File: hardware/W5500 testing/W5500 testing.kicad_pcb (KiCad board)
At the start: 2 copper layers, 34.4 x 55.3 mm, 42 parts, among them J4 Conn_01x08_Pin, J5 RJ45_Amphenol_RJMG1BD3B8K1ANR, Q4 MMBT5550L, Q5 MMBT5550L, U22 W5500, Y1 Crystal_GND24

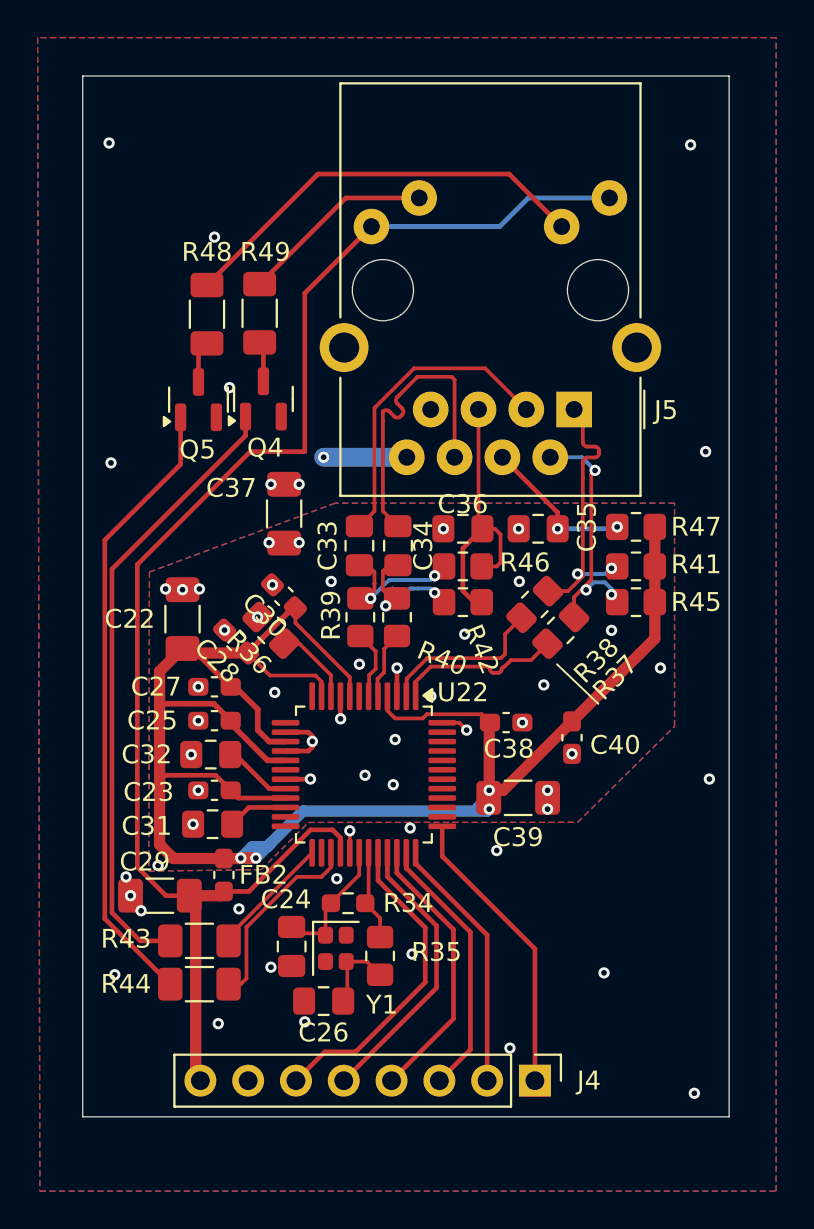
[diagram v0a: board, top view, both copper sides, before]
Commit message: mb v1.1 on da way
shuffled around stuff. review notes. made notes. glory to those who look forward and all that fuzz
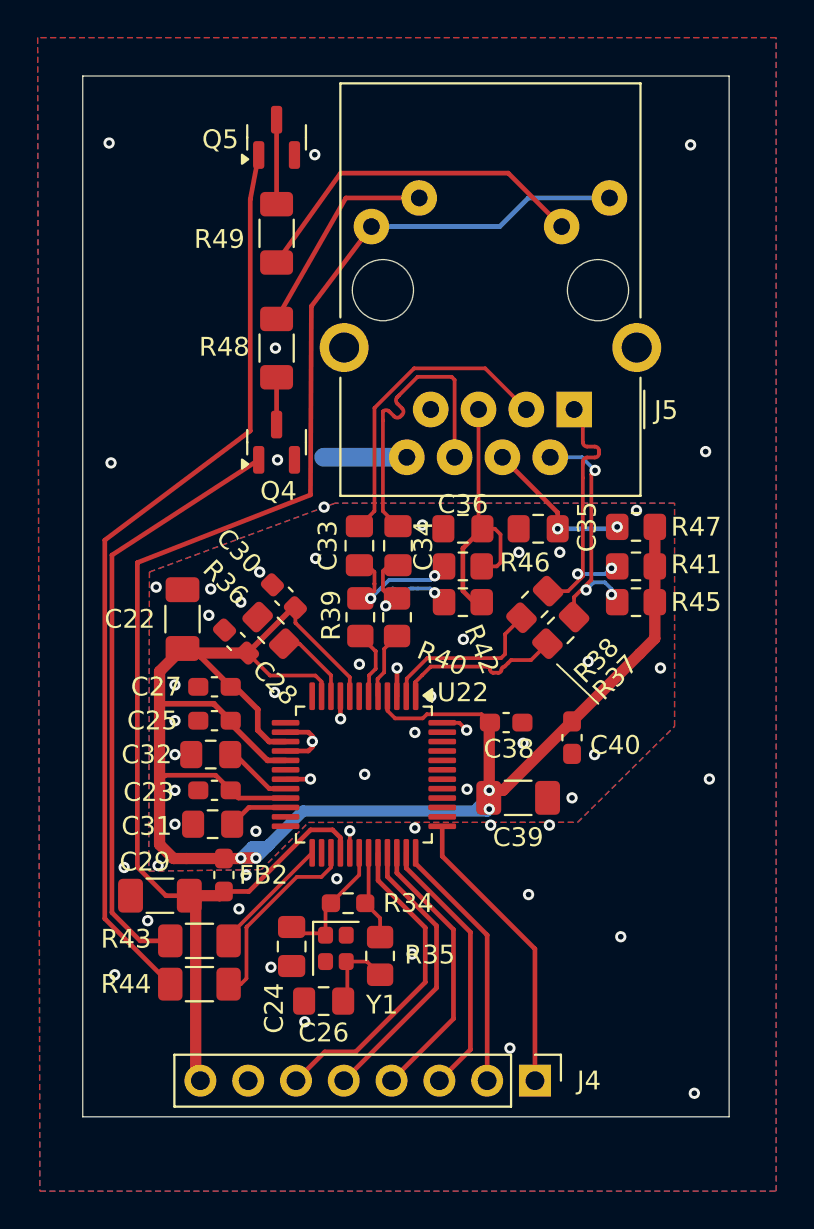
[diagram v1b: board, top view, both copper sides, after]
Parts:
- removed C37: 1n 2kV, Capacitor_SMD:C_1206_3216Metric_Pad1.33x1.80mm_HandSolder
- R35: value 0 -> 14.3
- moved Q5 14.5 mm to (115.8, 80.1)
- moved R49 5.67 mm to (115.8, 85.2), turned to 90 degrees
- moved Q4 2.40 mm to (115.8, 96.3)
- moved R48 2.06 mm to (115.8, 91.3)
- turned R35 to 90 degrees
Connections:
- R35 pad 1: Net-(U22-XO) -> Net-(C26-Pad1)
- R35 pad 2: Net-(C26-Pad1) -> Net-(U22-XO)
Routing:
- net Net-(Q5-B): track 33.2 -> 49.4 mm
- net Net-(J5-PadL3): track 22.5 -> 18.8 mm
- net Net-(Q5-C): track 2.24 -> 4.49 mm
- net Net-(Q4-B): track 33.0 -> 32.0 mm
- net Net-(J5-PadL2): track 10.4 -> 11.3 mm
- net /GND: vias 63 -> 60
